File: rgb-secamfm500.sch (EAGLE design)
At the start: 104 parts

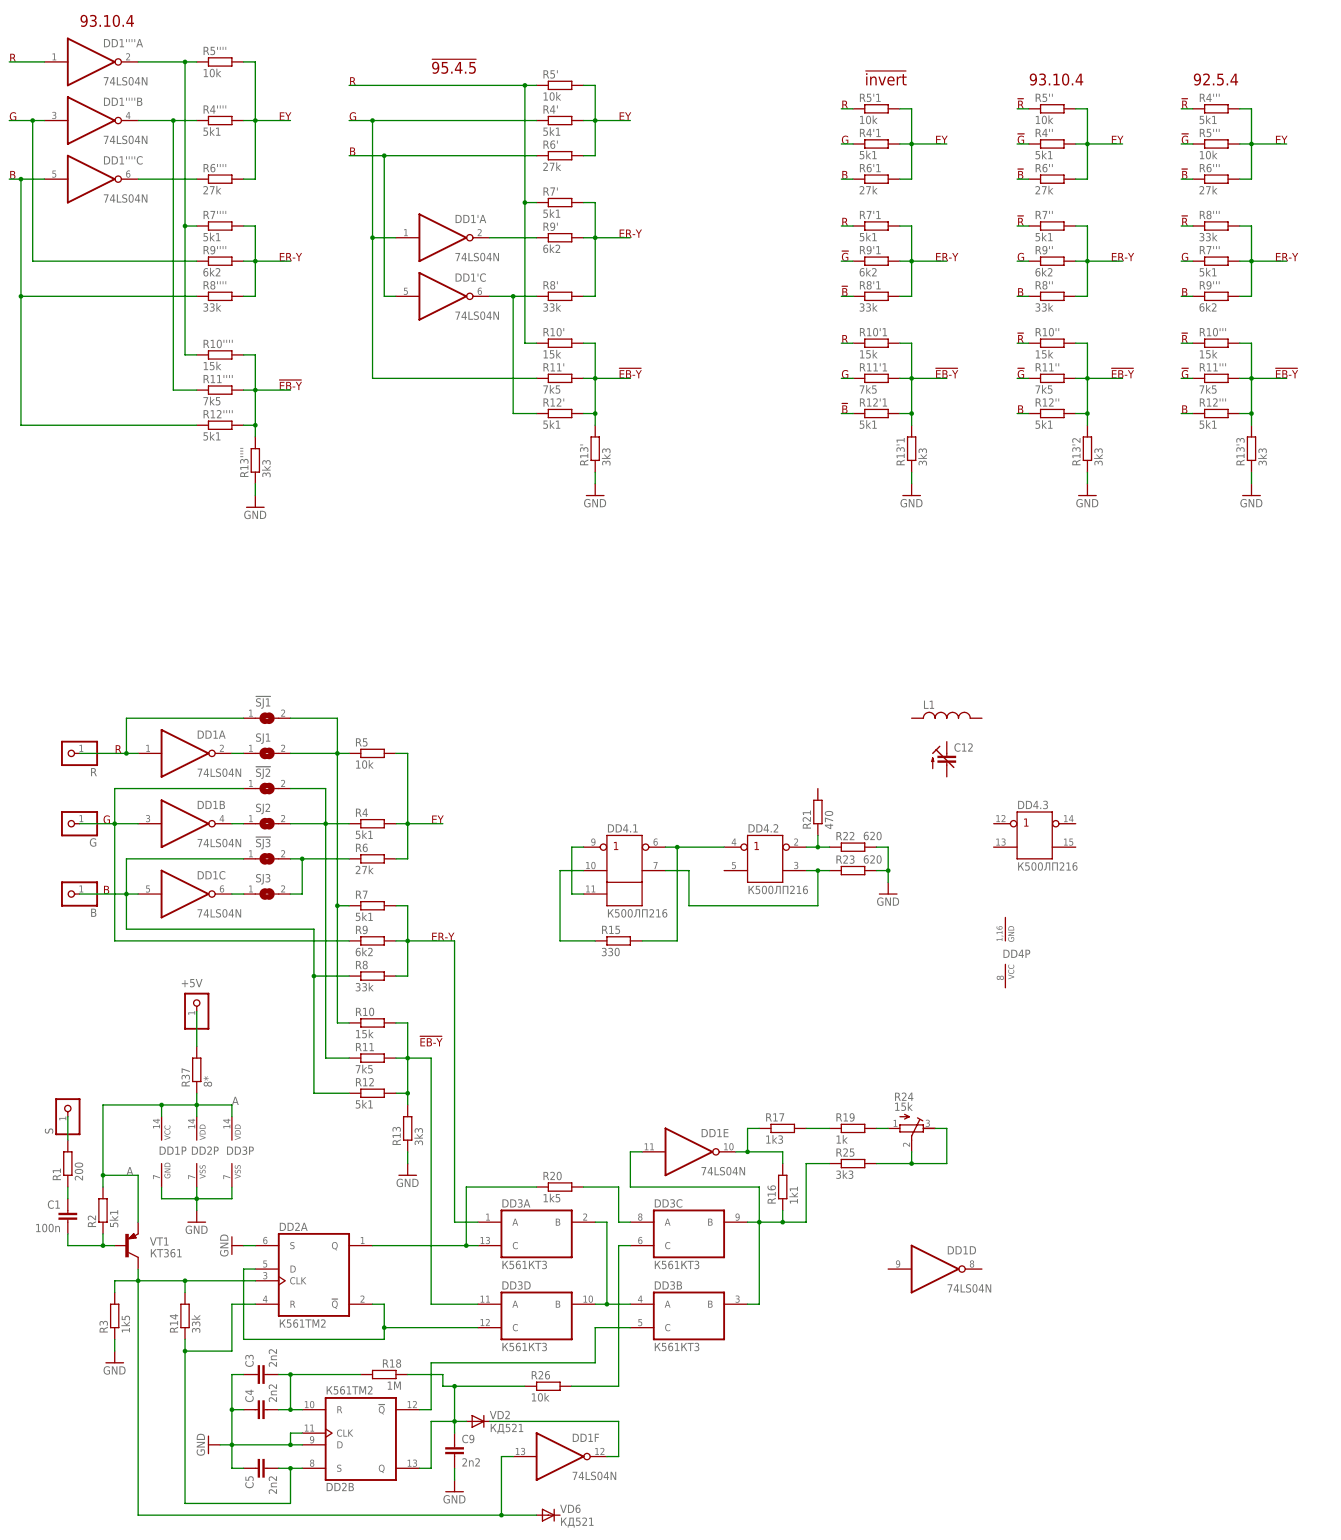
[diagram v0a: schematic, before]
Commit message: .
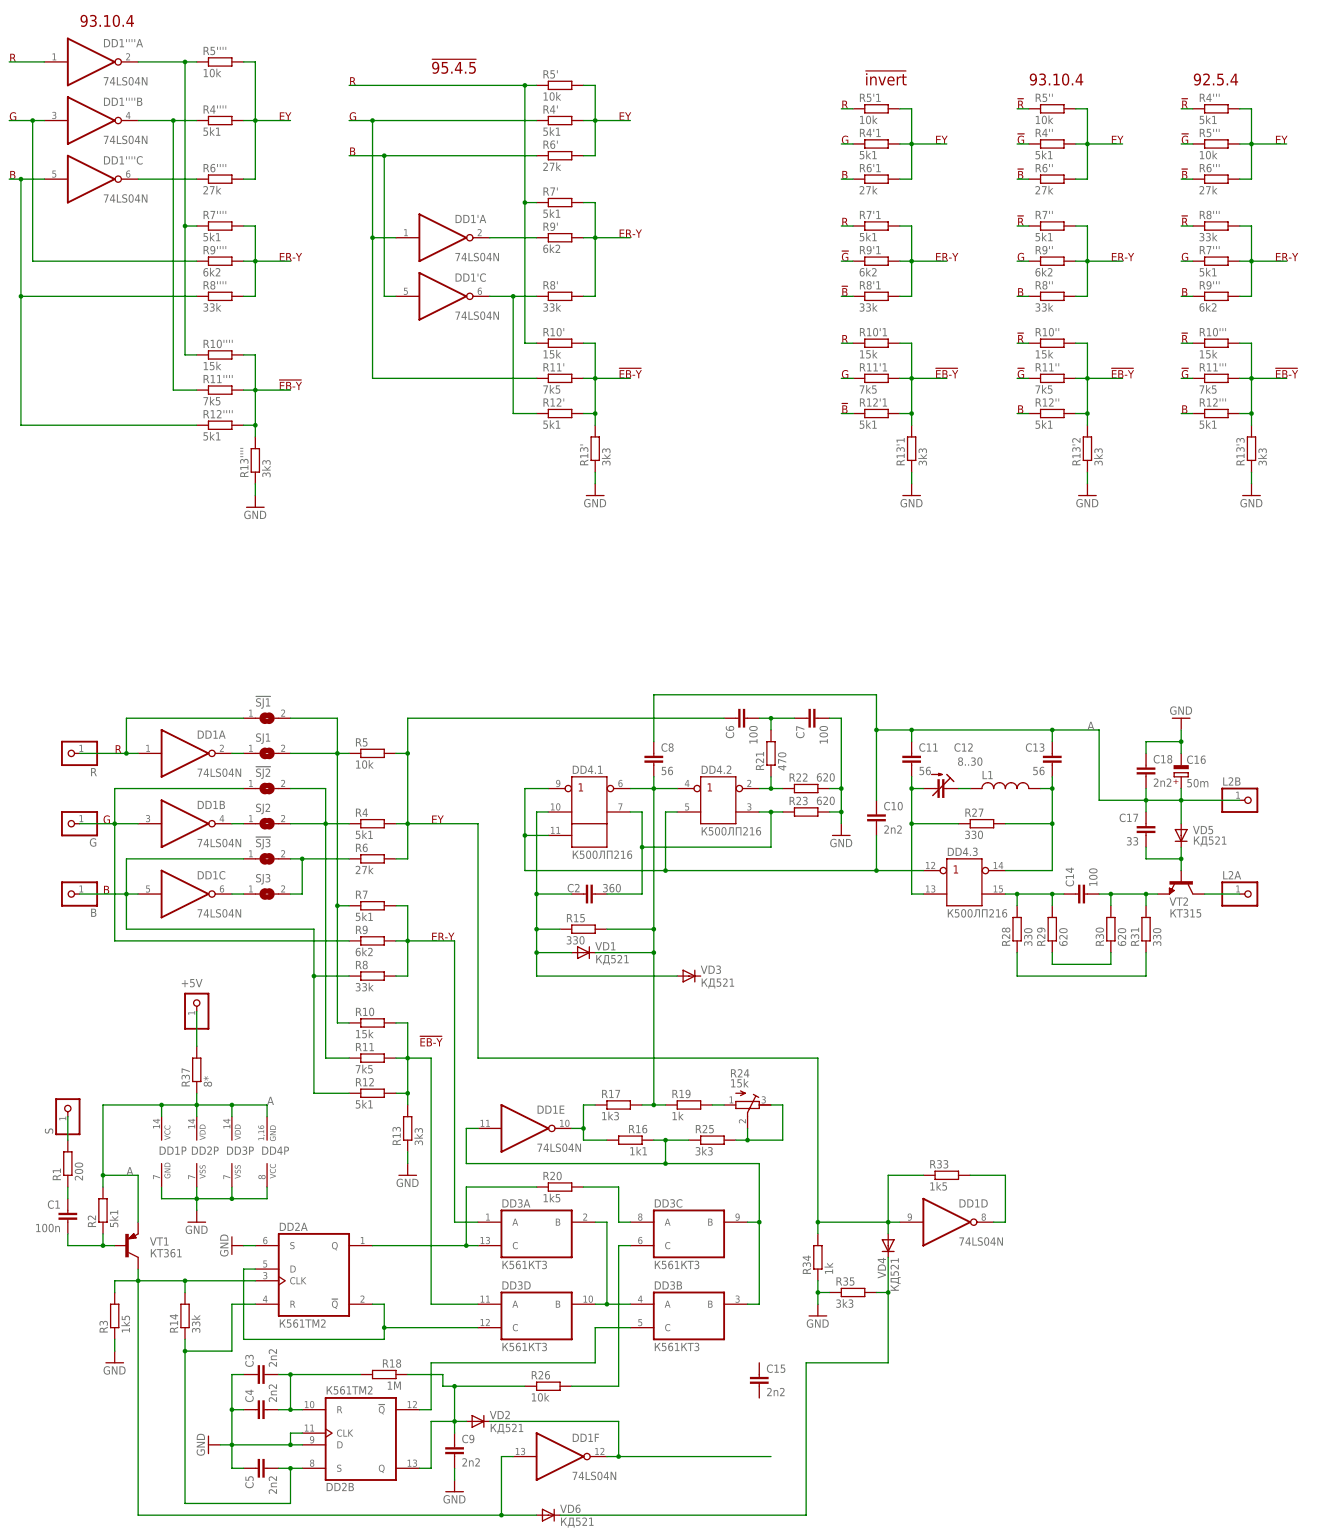
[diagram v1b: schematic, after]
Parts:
- added C10, C15, C18: 2n2, rcl:C-EUC0805K
- added C11, C13, C8: 56, rcl:C-EUC0805K
- added C14, C6, C7: 100, rcl:C-EUC0805K
- added C16: 50m, rcl:CPOL-EUE2.5-6
- added C17: 33, rcl:C-EUC0805K
- added C2: 360, rcl:C-EUC0805K
- added L2A, L2B: (no value), Разъёмы штырьковые 2.54мм:PINHD-1X1
- added R27, R28, R31: 330, rcl:R-EU_M0805
- added R29, R30: 620, rcl:R-EU_M0805
- added R33: 1k5, rcl:R-EU_M0805
- added R34: 1k, rcl:R-EU_M0805
- added R35: 3k3, rcl:R-EU_M0805
- added VD1, VD3, VD4, VD5: КД521, diode:DIODE-D-7.5
- added VT2: КТ315, m_transistor:BJT_NPN_TO-92_ECB
- C12: value (none) -> 8..30
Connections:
- new net N$100: L2A.1, VT2.C
- new net N$101: DD1D.O, R33.2
- new net N$102: R35.2, VD4.C, VD6.C
- new net N$91: C6.2, C7.1, R21.2
- new net N$92: C13.2, DD4.3.!OUT, L1.2, R27.2
- new net N$93: C12.E, L1.1
- new net N$94: C17.2, VD5.C, VT2.B
- new net N$95: C14.1, DD4.3.OUT, R28.2, R29.2
- new net N$96: C14.2, R30.2, R31.2, VT2.E
- new net N$97: R29.1, R30.1
- new net N$98: R28.1, R31.1
- net A: now also C10.1, C11.1, C13.1, C16.+, C17.1, C18.2, C8.1, DD4P.GND, L2B.1, VD5.A
- net GND: now also C16.-, C18.1, C7.2, DD4P.VCC, R34.1, R35.1
- net N$54: now also C6.1, DD1D.I, R33.1, R34.2, VD4.A
- net N$80: now also C8.2, DD4.1.!OUT, DD4.2.!IN, R15.2, VD1.C
- net N$85: now also C10.2, DD4.2.IN, DD4.3.!IN
- net N$86: now also C11.2, C12.A, DD4.3.IN, R27.1; no longer DD4.1.!OUT, DD4.2.!IN, R15.2
- net N$88: now also C2.2
- net N$89: now also C2.1, VD1.A, VD3.A
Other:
- note added: "RGBS to SECAM RF"
- moved on the sheet: C12, DD1D, DD1E, DD4.1, DD4.2, DD4.3, DD4P, L1, R15, R16, R17, R19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
